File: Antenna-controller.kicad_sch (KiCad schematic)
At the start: 17 parts, among them J1 Power_Supply, J3 SPI_Conn, M1 Motor_DC, Q1 BD138, Q2 BD137, Q3 BD138, Q4 BD137, U1 MCT6, U2 generic_imu, U3 ADG3300

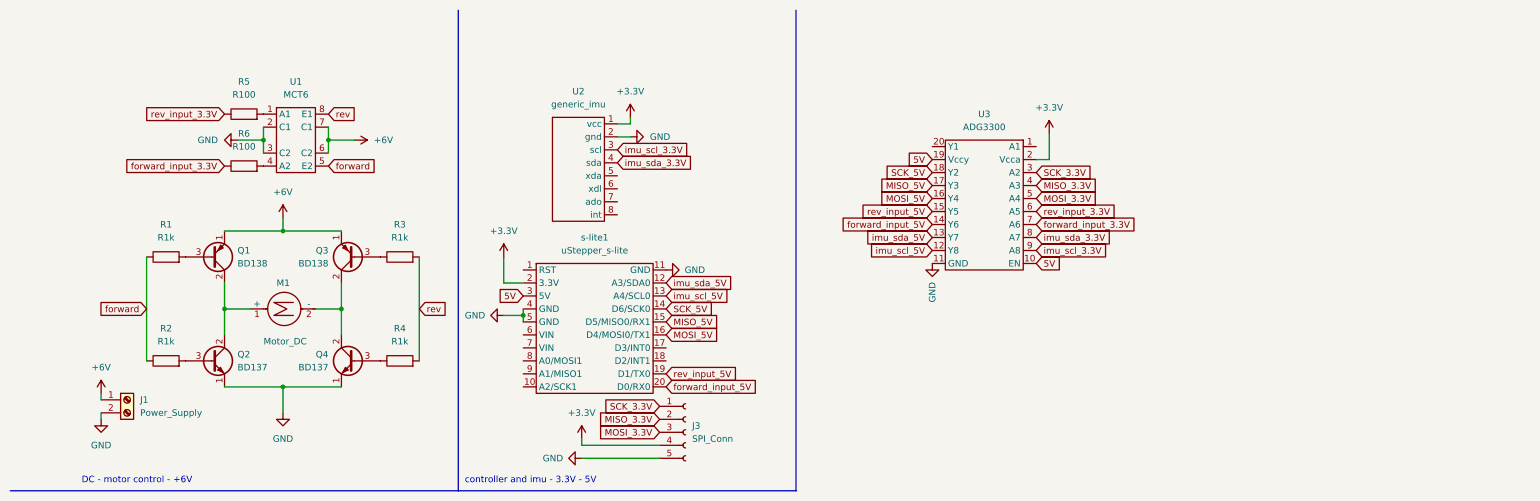
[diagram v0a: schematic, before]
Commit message: idk doing a backup
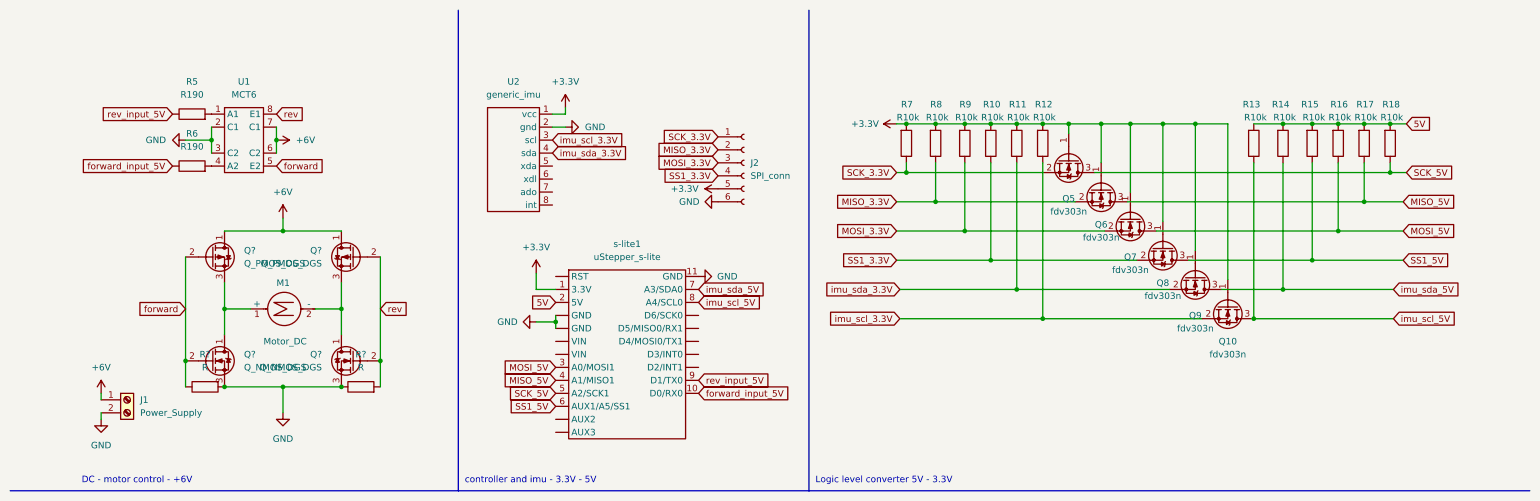
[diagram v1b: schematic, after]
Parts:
- removed J3: SPI_Conn, Connector_PinHeader_1.00mm:PinHeader_1x05_P1.00mm_Horizontal, symbol Connector:Conn_01x05_Female
- removed Q1, Q3: BD138, Package_TO_SOT_THT:TO-126-3_Vertical, symbol Transistor_BJT:BD138
- removed Q2, Q4: BD137, Package_TO_SOT_THT:TO-126-3_Vertical, symbol Transistor_BJT:BD137
- removed R1, R2, R3, R4: R1k, Resistor_THT:R_Axial_DIN0207_L6.3mm_D2.5mm_P10.16mm_Horizontal, symbol Device:R
- removed U3: ADG3300, ab2_tssop:AB2_TSSOP20, symbol Logic_LevelTranslator:ADG3300
- added J2: SPI_conn, Connector_PinHeader_1.27mm:PinHeader_1x06_P1.27mm_Horizontal, symbol Connector:Conn_01x06_Female
- added Q10, Q5, Q6, Q7, Q8, Q9: fdv303n, Package_TO_SOT_SMD:SOT-23_Handsoldering, symbol Device:Q_NMOS_GSD
- added Q? (x2): Q_PMOS_DGS, symbol Device:Q_PMOS_DGS
- added Q? (x2): Q_NMOS_DGS, symbol Device:Q_NMOS_DGS
- added R10, R11, R12, R13, R14, R15, R16, R17, R18, R7, R8, R9: R10k, Resistor_THT:R_Axial_DIN0207_L6.3mm_D2.5mm_P10.16mm_Horizontal, symbol Device:R
- added R? (x2): R, symbol Device:R
- R5, R6: value R100 -> R190
- U2: footprint Connector_PinHeader_1.27mm:PinHeader_1x08_P1.27mm_Vertical -> Connector_PinHeader_1.27mm:PinHeader_1x08_P1.27mm_Horizontal
- s-lite1: footprint (none) -> Connector_PinHeader_1.27mm:PinHeader_1x11_P1.27mm_Horizontal
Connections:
- net forward_input_3.3V is gone; now on net forward_input_5V: R6.1
- net rev_input_3.3V is gone; now on net rev_input_5V: R5.1
- net +3V3: now also s-lite1.1 (3.3V), J2.5 (Pin_5), Q10.1 (G), Q5.1 (G), Q6.1 (G), Q7.1 (G), Q8.1 (G), Q9.1 (G), R10.2, R11.2, R12.2, R7.2, R8.2, R9.2; no longer s-lite1.2 (3.3V)
- net +6V: now also Q?.1 (D), Q?.1 (D)
- net 5V: now also s-lite1.2 (5V), R13.2, R14.2, R15.2, R16.2, R17.2, R18.2; no longer s-lite1.3 (5V)
- net GND: now also s-lite1. (VIN), J2.6 (Pin_6), Q?.3 (S), Q?.3 (S), R?.1, R?.2; no longer s-lite1.4 (GND), s-lite1.5 (GND)
- net MISO_3.3V: now also J2.2 (Pin_2), Q6.2 (S), R8.1
- net MISO_5V: now also s-lite1.4 (A1/MISO1), Q6.3 (D), R17.1; no longer s-lite1.15 (D5/MISO0/RX1)
- net MOSI_3.3V: now also J2.3 (Pin_3), Q7.2 (S), R9.1
- net MOSI_5V: now also s-lite1.3 (A0/MOSI1), Q7.3 (D), R16.1; no longer s-lite1.16 (D4/MOSI0/TX1)
- net SCK_3.3V: now also J2.1 (Pin_1), Q5.2 (S), R7.1
- net SCK_5V: now also s-lite1.5 (A2/SCK1), Q5.3 (D), R18.1; no longer s-lite1.14 (D6/SCK0)
- net forward: now also Q?.2 (G), Q?.2 (G), R?.1
- net forward_input_5V: now also s-lite1.10 (D0/RX0); no longer s-lite1.20 (D0/RX0)
- net imu_scl_3.3V: now also Q10.2 (S), R12.1
- net imu_scl_5V: now also s-lite1.8 (A4/SCL0), Q10.3 (D), R13.1; no longer s-lite1.13 (A4/SCL0)
- net imu_sda_3.3V: now also Q9.2 (S), R11.1
- net imu_sda_5V: now also s-lite1.7 (A3/SDA0), Q9.3 (D), R14.1; no longer s-lite1.12 (A3/SDA0)
- net rev: now also Q?.2 (G), Q?.2 (G), R?.2
- net rev_input_5V: now also s-lite1.9 (D1/TX0); no longer s-lite1.19 (D1/TX0)
- net SS1_5V: now reaches s-lite1.6 (AUX1/A5/SS1)
- net SS1_5V: now also Q8.3 (D), R15.1
- net at M1.1 (+): now also Q?.1 (D), Q?.3 (S)
- net at M1.2 (-): now also Q?.1 (D), Q?.3 (S)
- new net SS1_3.3V: J2.4 (Pin_4), Q8.2 (S), R10.1
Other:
- note added: "Logic level converter 5V - 3.3V"
- moved on the sheet: R5, R6, U1, U2
